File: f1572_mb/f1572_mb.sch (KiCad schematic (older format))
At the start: 40 parts, among them Q1 MMBT3904, Q2 MMBT3904, Q3 MMBT3904, SW1 power, SW2 ~reset, U1 PIC12F1572

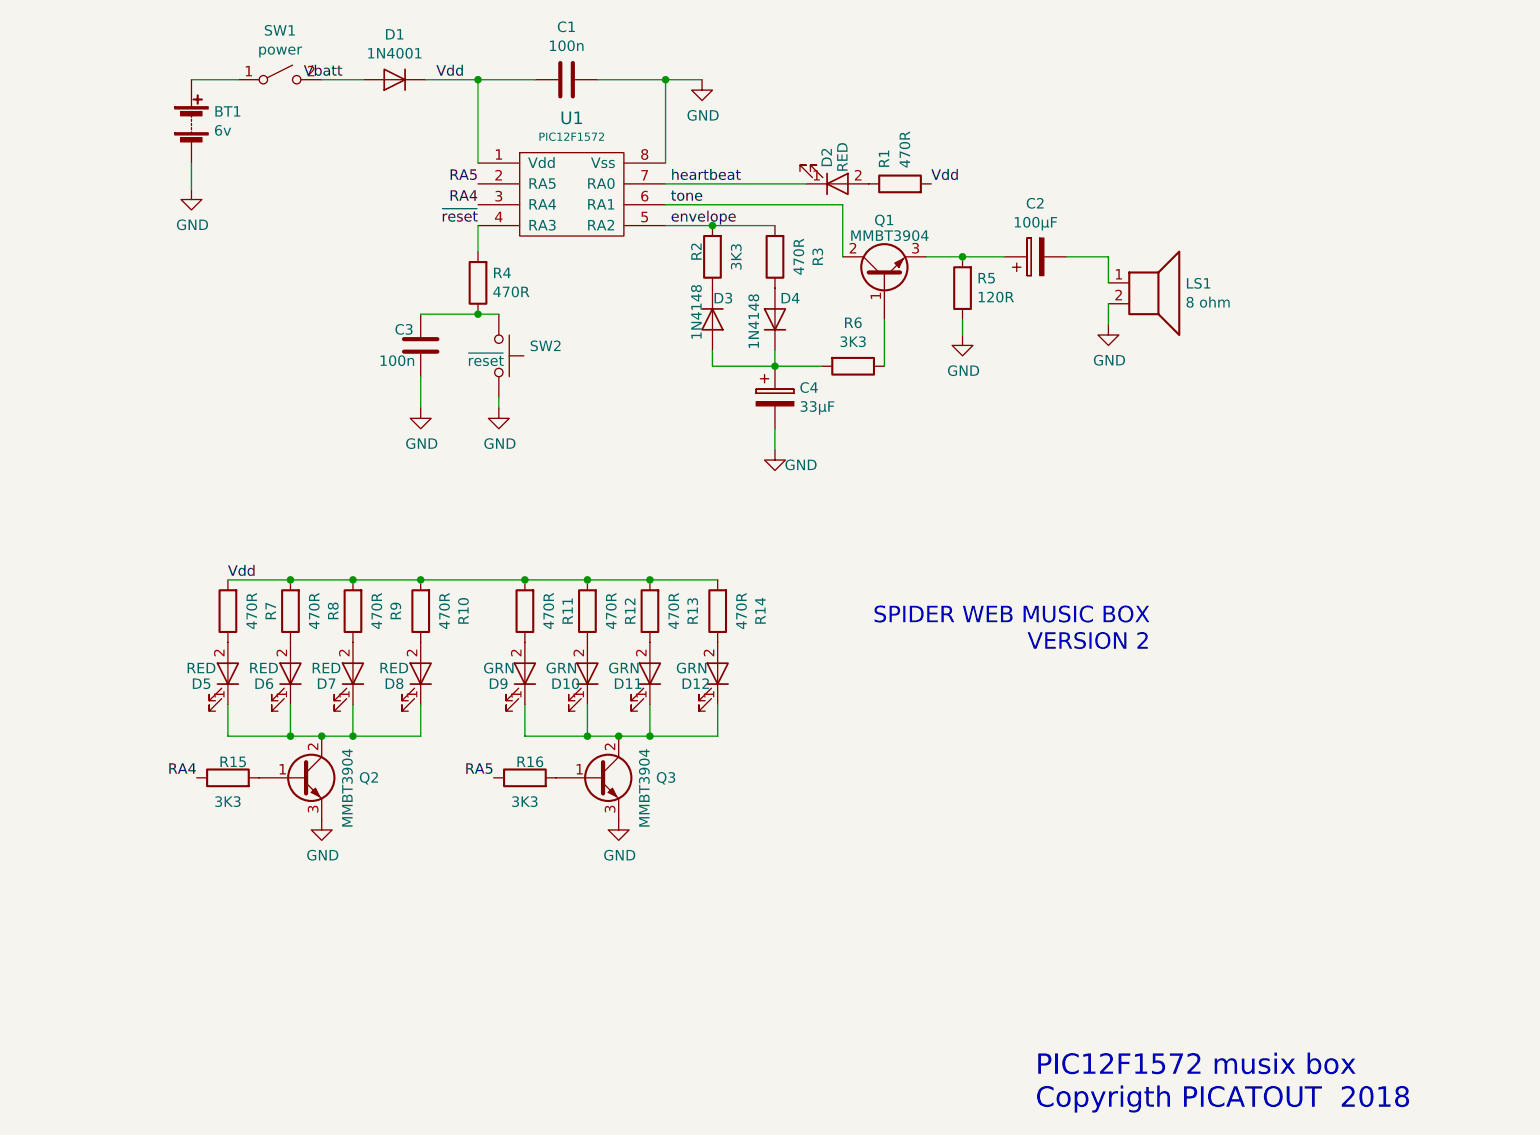
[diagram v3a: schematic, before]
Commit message: removed version 1
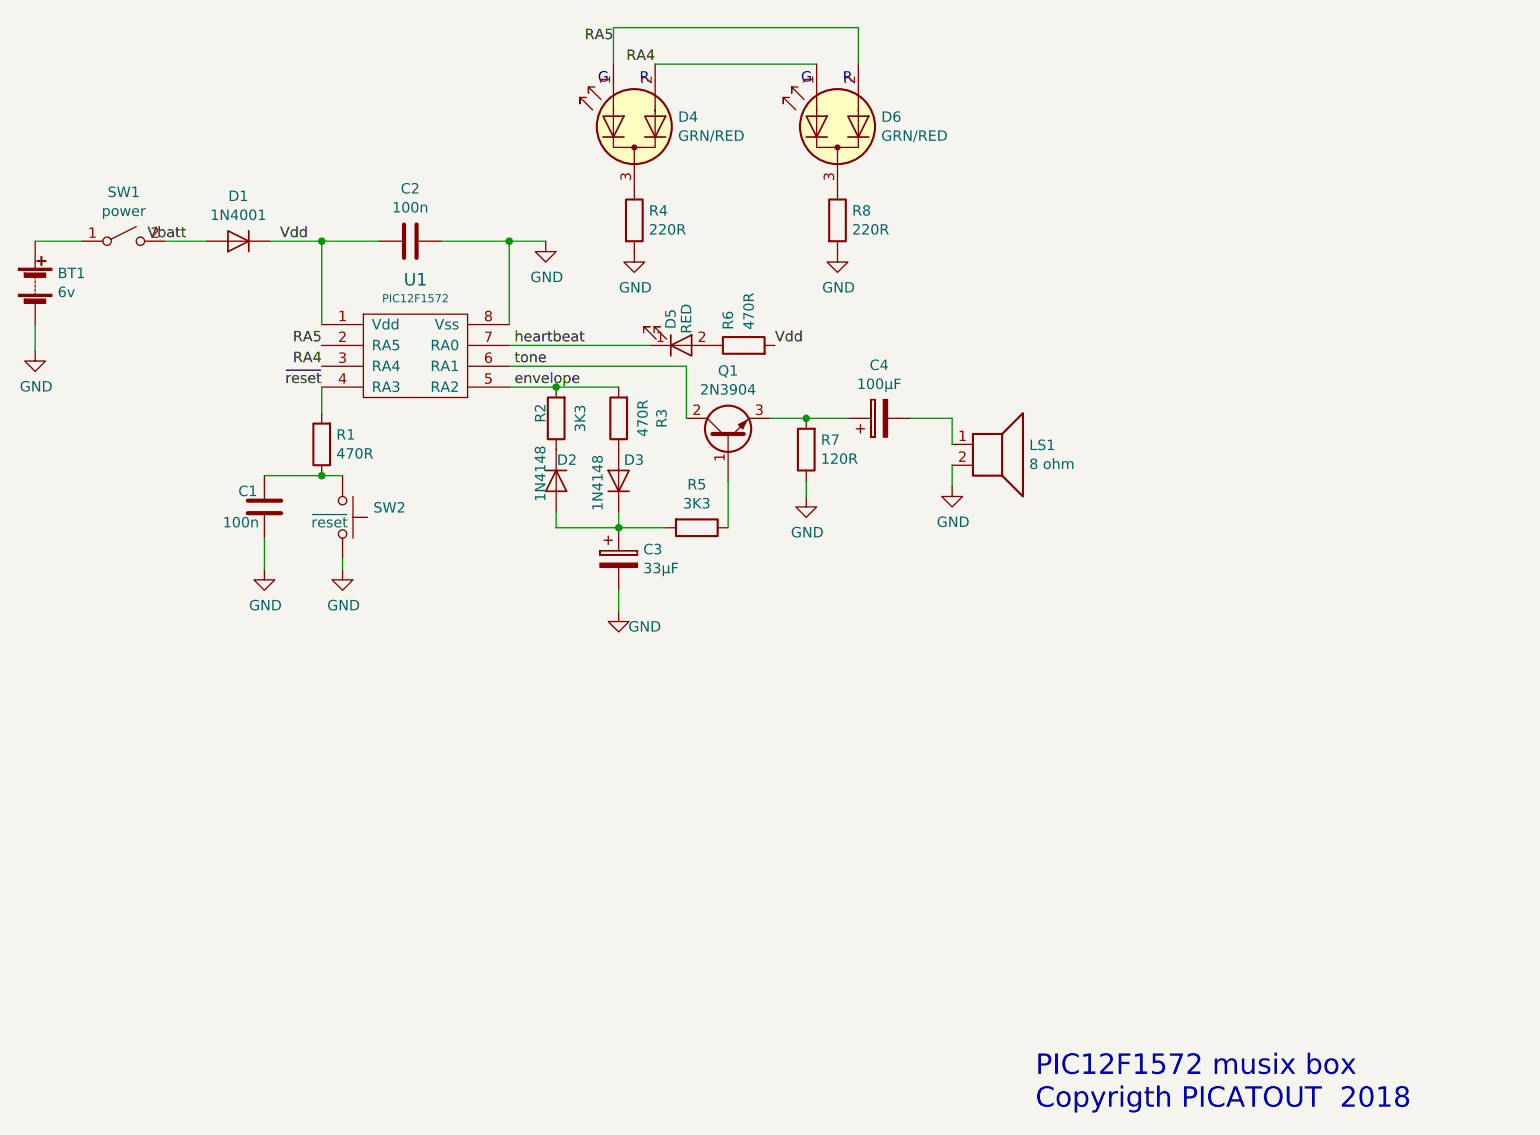
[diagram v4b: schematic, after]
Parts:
- removed D10, D11, D12, D9: GRN, LEDs:LED_0805, symbol device:LED
- removed D5, D6, D7, D8: RED, LEDs:LED_0805, symbol device:LED
- removed Q2, Q3: MMBT3904, TO_SOT_Packages_SMD:SOT-23, symbol device:Q_NPN_BCE
- removed R10, R11, R12, R13, R14, R7, R9: 470R, Resistors_SMD:R_0805, symbol device:R
- removed R15, R16: 3K3, Resistors_SMD:R_0805, symbol device:R
- added D4, D6: GRN/RED, symbol device:LED_Dual_AAC
- added R4: 220R, symbol device:R
- C1: renamed from C3; footprint Capacitors_SMD:C_0805 -> (none)
- C2: renamed from C1; footprint Capacitors_SMD:C_0805 -> (none)
- D1, R3: footprint Diodes_SMD:D_0805 -> (none)
- D2: renamed from D3; footprint Diodes_SMD:D_0805 -> (none)
- D3: renamed from D4; footprint Diodes_SMD:D_0805 -> (none)
- D5: renamed from D2; footprint LEDs:LED_0805 -> (none)
- Q1: value MMBT3904 -> 2N3904; footprint TO_SOT_Packages_SMD:SOT-23 -> (none)
- R1: renamed from R4; footprint Resistors_SMD:R_1206 -> (none)
- R2: footprint Resistors_SMD:R_0805 -> (none)
- R5: renamed from R6; footprint Resistors_SMD:R_0805 -> (none)
- R6: renamed from R1; footprint Resistors_SMD:R_0805 -> (none)
- R7: renamed from R5; footprint Resistors_SMD:R_0805 -> (none)
- R8: value 470R -> 220R; footprint Resistors_SMD:R_0805 -> (none)
- U1: footprint SMD_Packages:SOIC-8-N -> (none)
- renumbered C4 to C3, C2 to C4
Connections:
- net GND: now also R8.2, R4.2
- net RA4: now also D4.2 (A2), D6.1 (A1)
- net RA5: now also D4.1 (A1), D6.2 (A2)
- net Vdd: no longer R8.2
- net at R8.1: now also D6.3 (K)
- new net: D4.3 (K), R4.1
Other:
- note added: "G\n"
- note added: "R"
- note removed: "SPIDER WEB MUSIC BOX\nVERSION 2"
- moved on the sheet: BT1, C1, C2, C3, C4, D1, D2, D3, D5, LS1, Q1, R1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
